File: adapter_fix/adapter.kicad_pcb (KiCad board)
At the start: 2 copper layers, 96 x 18 mm, 10 parts, among them J11 MALE, J12 FEMALE, J13 MALE, J14 STANDOFF, J15 STANDOFF, J16 STANDOFF

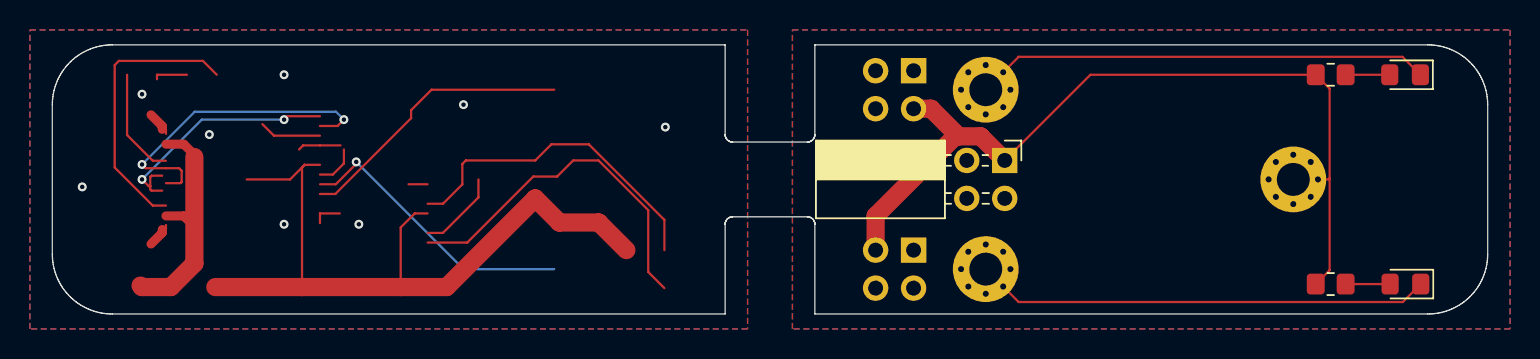
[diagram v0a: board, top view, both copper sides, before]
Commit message: Trace
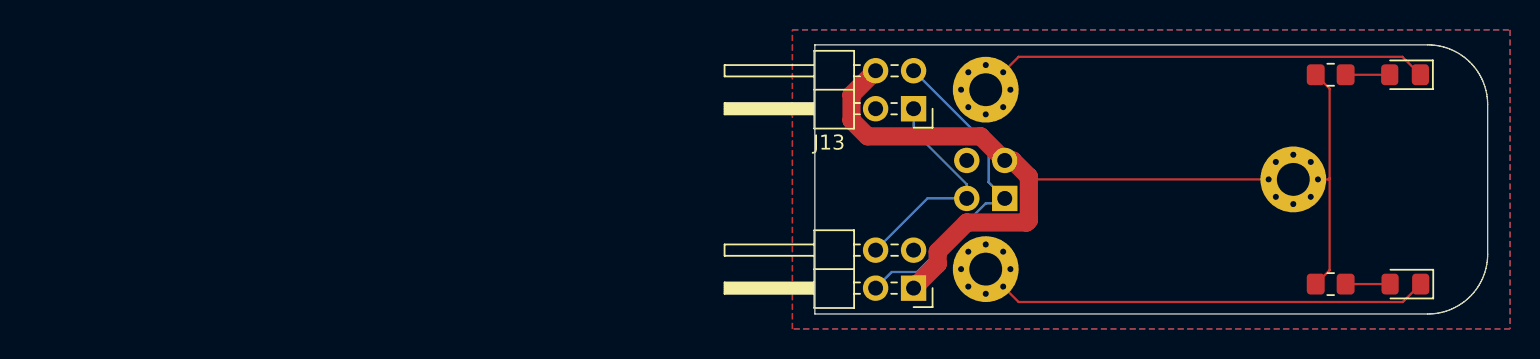
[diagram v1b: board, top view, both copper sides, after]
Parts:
- J11, J13: moved to F.Cu
- J12: moved to B.Cu
- moved J11 14.5 mm to (158.1, 112.3)
- moved J13 9.46 mm to (158.1, 100.3)
- moved J12 2.54 mm to (164.2, 106.3)
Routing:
- net +5VB: track 51.1 -> 0.00 mm
- net /Lower Board/TXD: track 24.1 -> 0.00 mm
- net /Lower Board/RXD: track 22.4 -> 0.00 mm
- net Net-(J11-Pad2): track 0.00 -> 22.2 mm
- net /Lower Board/D-: track 21.6 -> 0.00 mm, vias 2 -> 0
- net /Lower Board/RXLED: track 19.3 -> 0.00 mm, vias 1 -> 0
- net /Lower Board/VBUS: track 19.1 -> 0.00 mm
- net /Lower Board/TXLED: track 18.9 -> 0.00 mm
- net Net-(J6-PadB5): track 18.7 -> 0.00 mm
- net /Lower Board/D+: track 16.9 -> 0.00 mm, vias 2 -> 0
- net Net-(J11-Pad4): track 0.00 -> 15.0 mm
- net GNDB: track 14.4 -> 0.00 mm, vias 8 -> 0
- net +5V: track 58.0 -> 65.5 mm
- net Net-(J6-PadA5): track 7.34 -> 0.00 mm
- net /Lower Board/DTR: track 5.59 -> 0.00 mm
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- removed copper zone on B.Cu, net GNDB
- removed copper zone on F.Cu, net GNDB
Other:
- board size 96 x 18 mm -> 45 x 18 mm
